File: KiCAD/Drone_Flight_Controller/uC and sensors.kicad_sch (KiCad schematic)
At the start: 5 parts, among them U21 DPS368, U22 BNO055, U23 ESP32-WROOM-32

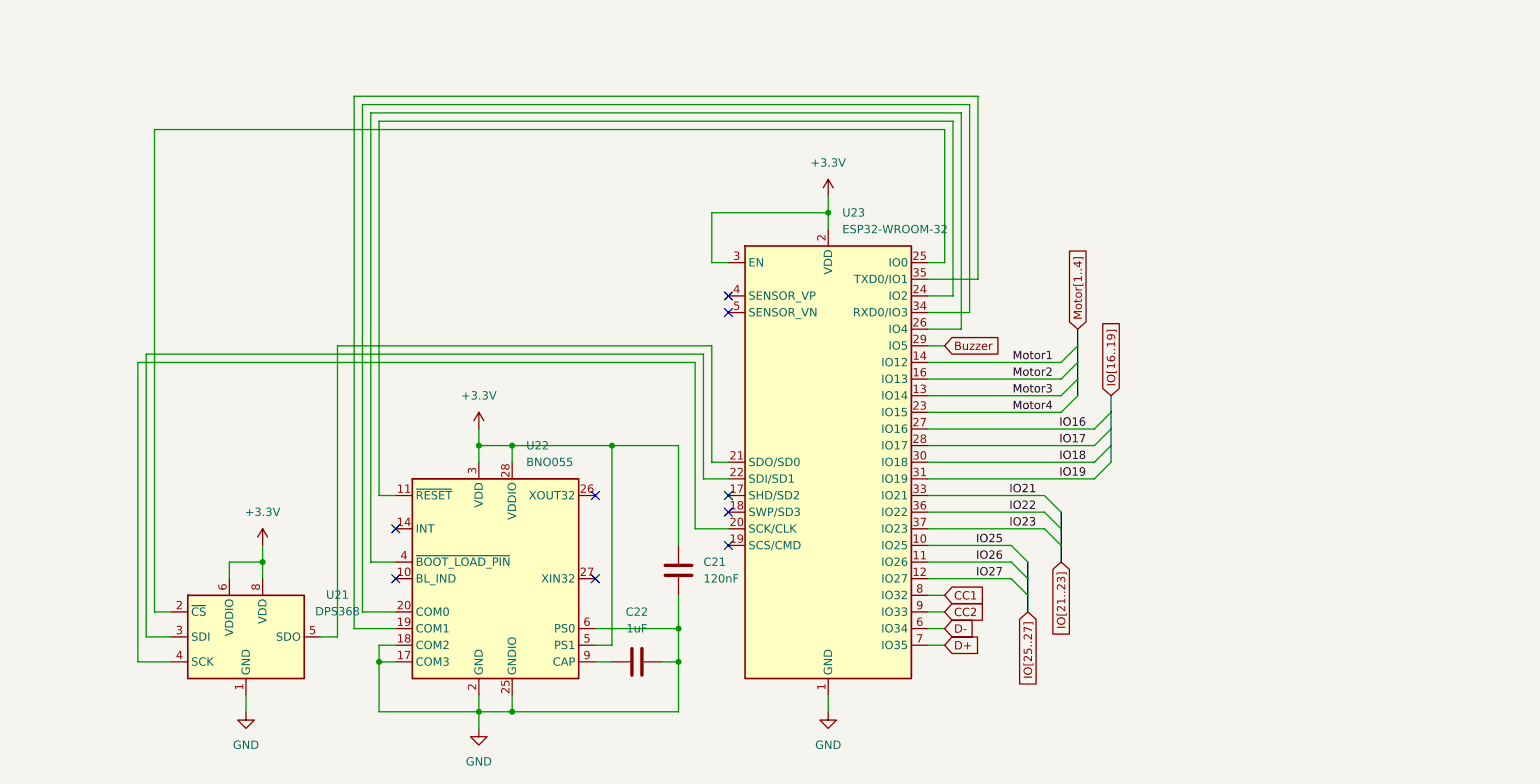
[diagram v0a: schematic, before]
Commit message: Add Programming
Add Programming
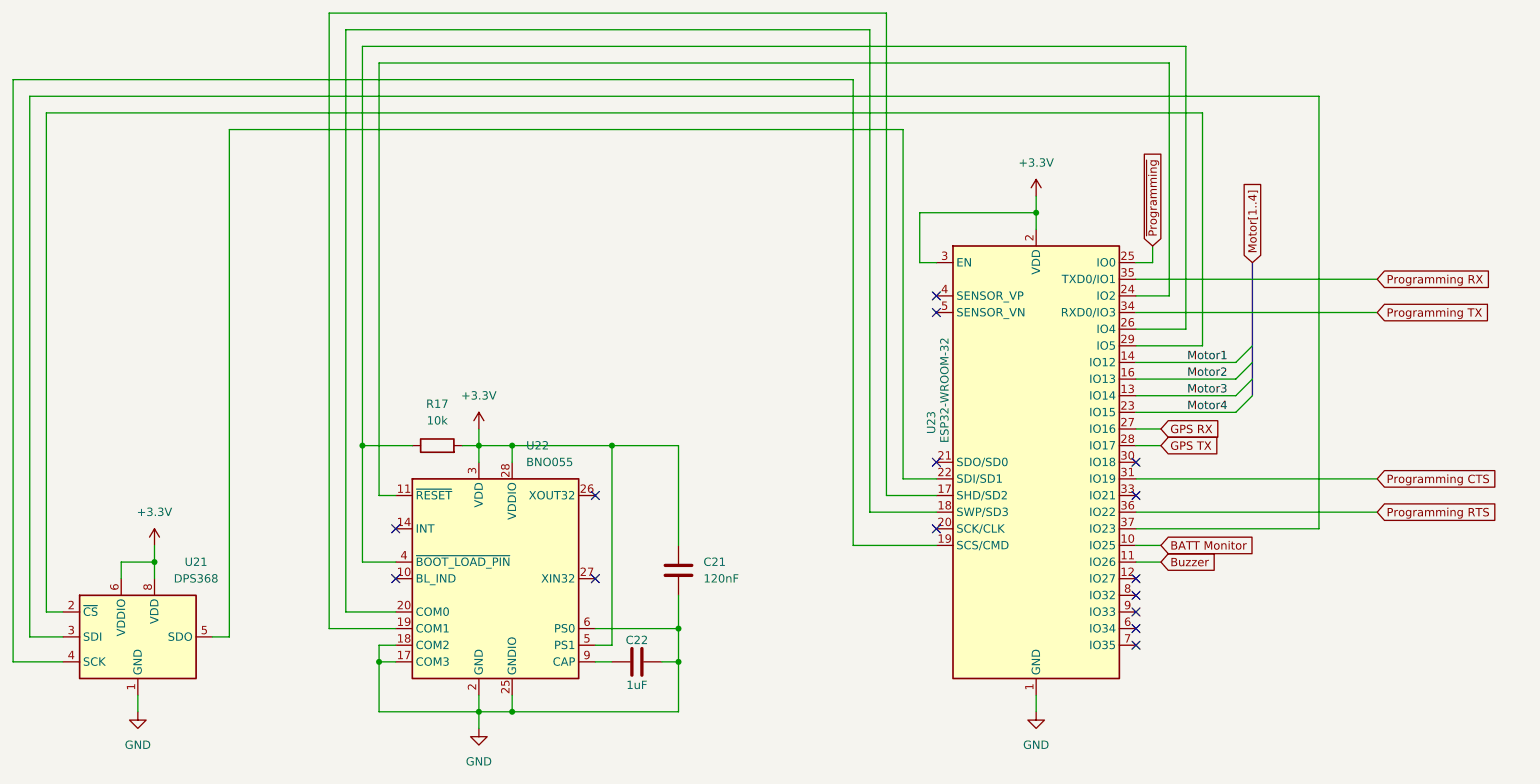
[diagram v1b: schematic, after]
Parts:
- added R17: 10k, Resistor_SMD:R_0805_2012Metric_Pad1.20x1.40mm_HandSolder, symbol Device:R
- C21: footprint (none) -> Capacitor_SMD:C_0805_2012Metric_Pad1.18x1.45mm_HandSolder; Link (none) -> https://www.mouser.at/ProductDetail/Vishay-Vitramon/VJ0805Y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
- C22: footprint (none) -> Capacitor_SMD:C_0805_2012Metric_Pad1.18x1.45mm_HandSolder; Link (none) -> https://www.mouser.at/ProductDetail/Samsung-Electro-Mechani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
- U21: footprint (none) -> Package_LGA:Bosch_LGA-8_2x2.5mm_P0.65mm_ClockwisePinNumbering
- U23: Link (none) -> /
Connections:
- net IO26 is gone; now on net Buzzer: U23.11 (IO26)
- net +3.3V: now also R17.2
- net Buzzer: no longer U23.29 (IO5)
- net at U23.17 (SHD/SD2): now also U22.19 (COM1)
- net at U23.18 (SWP/SD3): now also U22.20 (COM0)
- net at U23.19 (SCS/CMD): now also U21.4 (SCK)
- net at U23.20 (SCK/CLK): no longer U21.4 (SCK)
- net at U23.21 (SDO/SD0): no longer U21.5 (SDO)
- net at U23.22 (SDI/SD1): now also U21.5 (SDO); no longer U21.3 (SDI)
- net at U21.2 (~{CS}): now also U23.29 (IO5); no longer U23.25 (IO0)
- net at U22.4 (~{BOOT_LOAD_PIN}), U23.26 (IO4): now also R17.1
- net Programming TX: now reaches U23.34 (RXD0/IO3)
- net Programming TX: no longer U22.20 (COM0)
- net Programming RX: now reaches U23.35 (TXD0/IO1)
- net Programming RX: no longer U22.19 (COM1)
- net CC1: no longer names the net of U23.8 (IO32)
- net CC2: no longer names the net of U23.9 (IO33)
- net D+: no longer names the net of U23.7 (IO35)
- net D-: no longer names the net of U23.6 (IO34)
- net IO16 renamed GPS RX
- net IO17 renamed GPS TX
- net IO18: no longer names the net of U23.30 (IO18)
- net IO19 renamed Programming CTS
- net IO21: no longer names the net of U23.33 (IO21)
- net IO22 renamed Programming RTS
- net IO23: no longer names the net of U23.37 (IO23)
- net IO23: now also U21.3 (SDI)
- net IO25 renamed BATT Monitor
- net IO27: no longer names the net of U23.12 (IO27)
- new net ~{Programming}: U23.25 (IO0)
- no-connect marks 9 -> 15
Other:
- moved on the sheet: U21, U23
